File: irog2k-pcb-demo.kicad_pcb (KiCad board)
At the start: 2 copper layers, 42.9 x 60.9 mm, 20 parts, among them SW1 SW_Push, U1 ATmega32U4-AU, Y1 16MHz

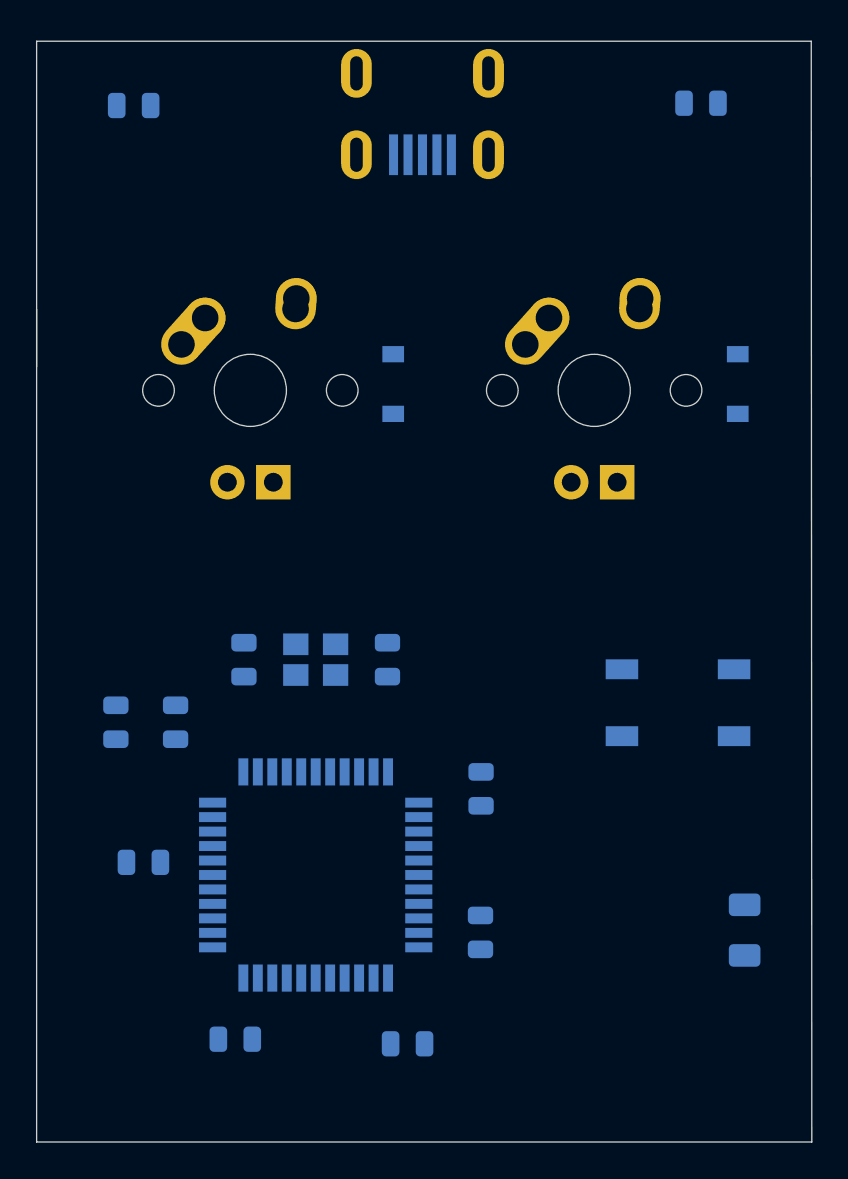
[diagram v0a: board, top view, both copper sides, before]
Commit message: pcb (finished)
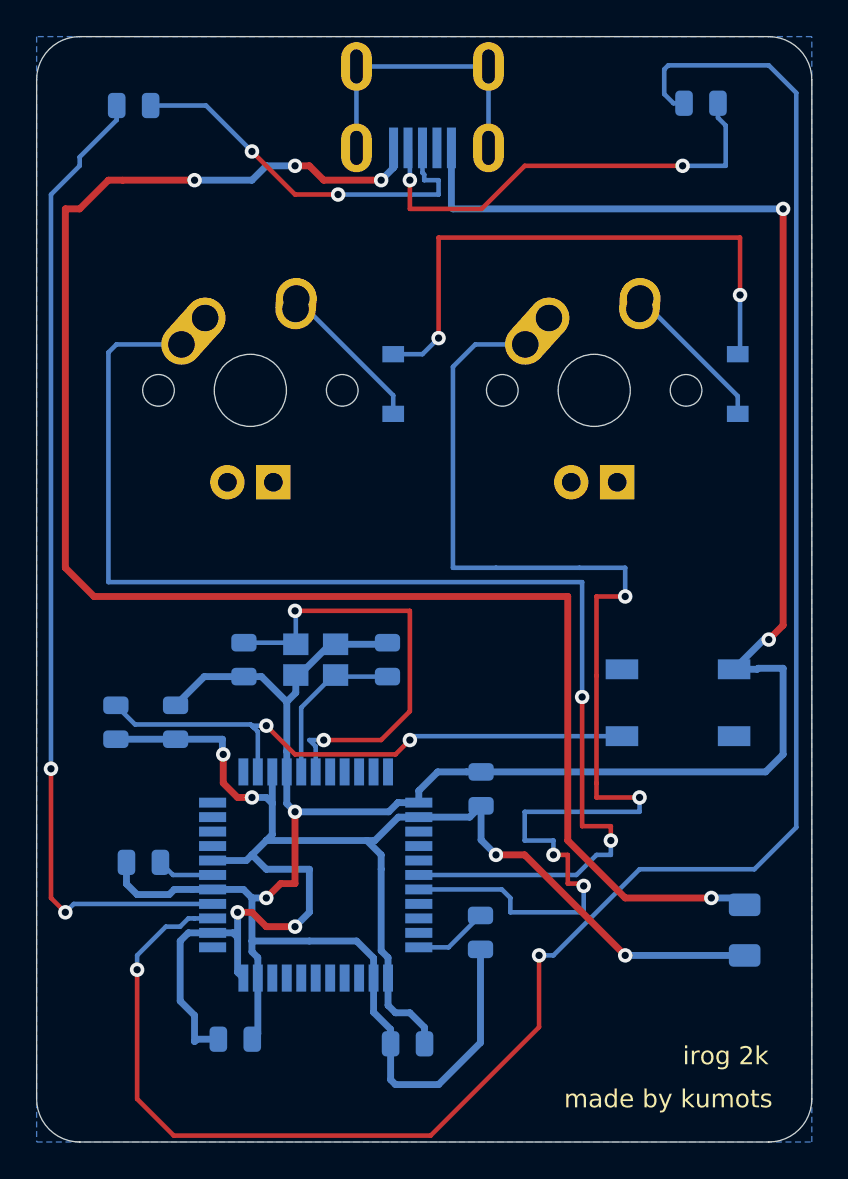
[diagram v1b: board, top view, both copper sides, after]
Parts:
- moved USB1 0.38 mm to (103.1, 46.1)
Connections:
- net Net-(F1-Pad2) renamed VCC
- MX1 pad 1: Net-(MX1-Pad1) -> COL0
- MX2 pad 1: Net-(MX2-Pad1) -> COL1
- U1 pad 28: Net-(U1-Pad28) -> COL0
- U1 pad 29: Net-(U1-Pad29) -> COL1
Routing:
- net GND: track 0.00 -> 154.6 mm, vias 0 -> 4
- net Net-(R1-Pad1): track 0.00 -> 110.9 mm, vias 0 -> 2
- net VCC: track 0.00 -> 93.9 mm, vias 0 -> 4
- net +5V: track 0.00 -> 88.7 mm, vias 0 -> 6
- net COL0: track 0.00 -> 70.9 mm, vias 0 -> 2
- net COL1: track 0.00 -> 67.8 mm, vias 0 -> 4
- net Net-(R2-Pad1): track 0.00 -> 54.8 mm, vias 0 -> 2
- net Net-(R3-Pad2): track 0.00 -> 32.4 mm, vias 0 -> 2
- net ROW0: track 0.00 -> 31.6 mm, vias 0 -> 2
- net D-: track 0.00 -> 25.5 mm, vias 0 -> 2
- net Net-(C3-Pad1): track 0.00 -> 24.8 mm, vias 0 -> 2
- net D+: track 0.00 -> 21.5 mm, vias 0 -> 2
- net Net-(USB1-Pad6): track 0.00 -> 16.3 mm
- net Net-(C4-Pad1): track 0.00 -> 9.11 mm
- net Net-(D2-Pad2): track 0.00 -> 8.42 mm
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- added copper zone on B.Cu, net GND
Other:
- board size 42.9 x 60.9 mm -> 42.9 x 61.1 mm
- net class Default: trace_width 0.25 -> 0.254
- net class Power added: clearance 0.2, trace_width 0.381, via_dia 0.8, via_drill 0.4
- board text added: "irog 2k"
- board text added: "made by kumots"
